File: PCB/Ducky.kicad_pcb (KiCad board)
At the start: 2 copper layers, 34.5 x 94.5 mm, 4 parts, among them J1 Conn_01x22_Socket, J2 Conn_01x22_Socket, U1 ESP32-S3

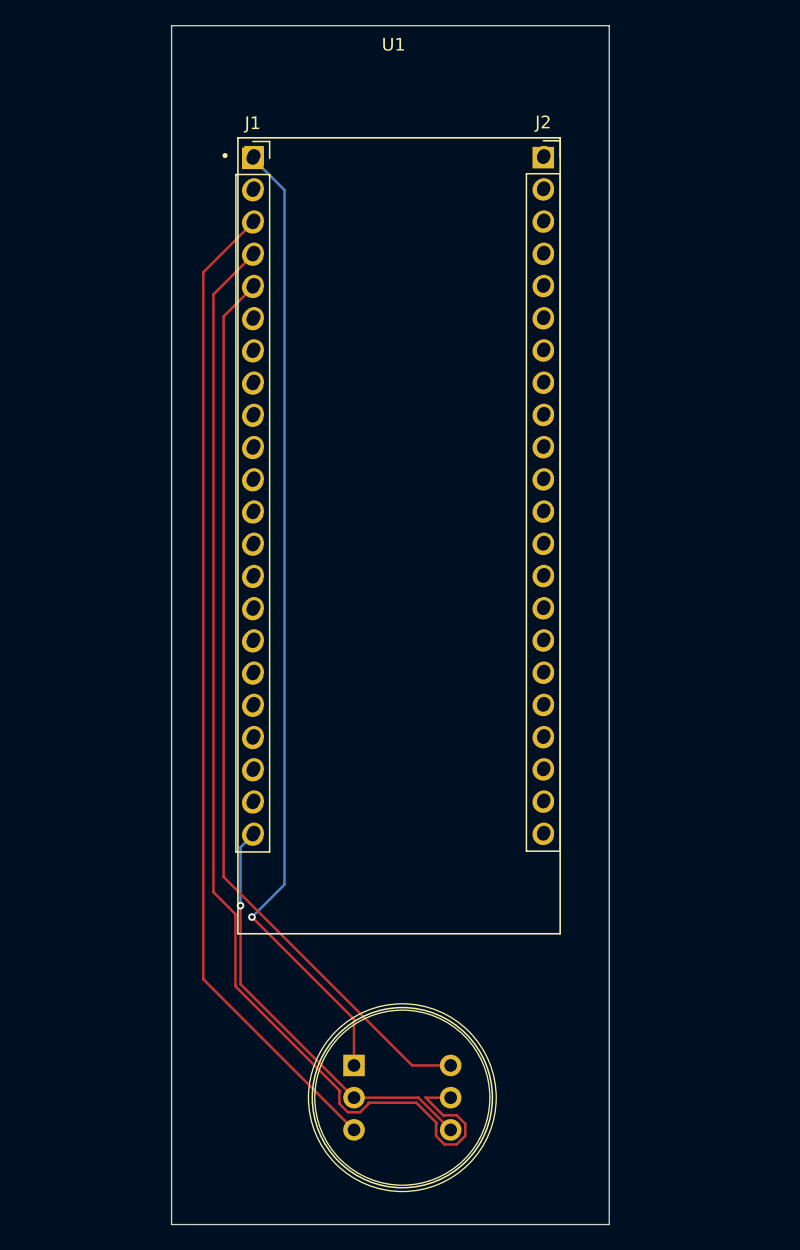
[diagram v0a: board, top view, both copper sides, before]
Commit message: I am organzing my folders and files
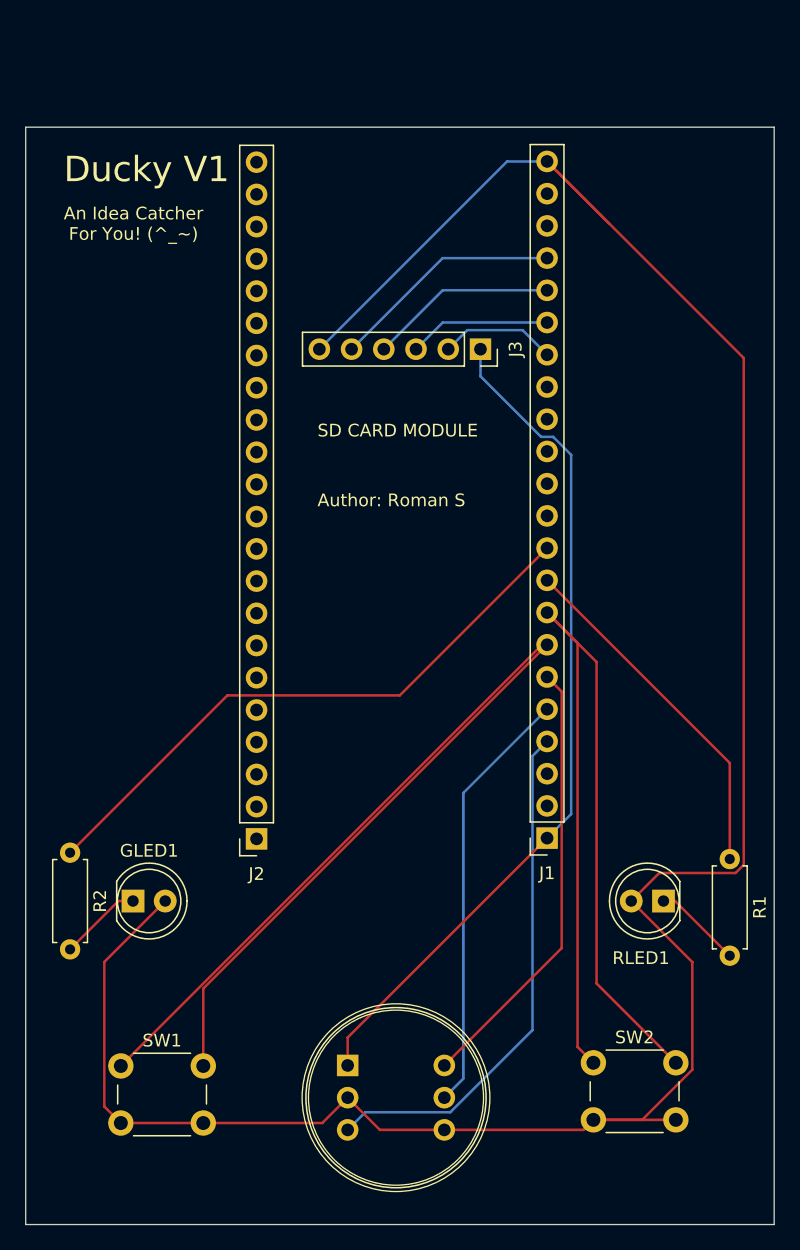
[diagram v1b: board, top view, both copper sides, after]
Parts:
- removed U1: ESP32-S3, ESP32-S3-DEVKITC-1-N8R2:XCVR_ESP32-S3-DEVKITC-1-N8R2
- added GLED1: LED, LED_THT:LED_D5.0mm, F.Cu at (130.5, 97.0)
- added J3: Conn_01x06_Socket, Connector_PinSocket_2.54mm:PinSocket_1x06_P2.54mm_Vertical, F.Cu at (157.8, 53.5)
- added R1: R, Resistor_THT:R_Axial_DIN0207_L6.3mm_D2.5mm_P7.62mm_Horizontal, F.Cu at (177.5, 93.7)
- added R2: R, Resistor_THT:R_Axial_DIN0207_L6.3mm_D2.5mm_P7.62mm_Horizontal, F.Cu at (125.5, 93.2)
- added RLED1: LED, LED_THT:LED_D5.0mm, F.Cu at (172.3, 97.0)
- added SW1: On/Off Button, Button_Switch_THT:SW_PUSH_6mm_H7.3mm, F.Cu at (129.5, 110.0)
- added SW2: Recording/Stop Recording Button, Button_Switch_THT:SW_PUSH_6mm_H7.3mm, F.Cu at (166.8, 109.8)
- moved J1 58.4 mm to (163.1, 92.0), turned to 180 degrees
- moved J2 58.3 mm to (140.2, 92.1), turned to 180 degrees
- moved M1 0.50 mm to (151.2, 112.5)
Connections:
- J1 pad 10: unconnected-(J1-Pin_10-Pad10) -> /GLED
- J1 pad 16: unconnected-(J1-Pin_16-Pad16) -> /CS
- J1 pad 17: unconnected-(J1-Pin_17-Pad17) -> /MOSI
- J1 pad 18: unconnected-(J1-Pin_18-Pad18) -> /CLK
- J1 pad 19: unconnected-(J1-Pin_19-Pad19) -> /MISO
- J1 pad 3: /SD -> unconnected-(J1-Pin_3-Pad3)
- J1 pad 4: /WS -> /SD
- J1 pad 5: /SCK -> /WS
- J1 pad 6: unconnected-(J1-Pin_6-Pad6) -> /SCK
- J1 pad 7: unconnected-(J1-Pin_7-Pad7) -> /On/Off Btn
- J1 pad 8: unconnected-(J1-Pin_8-Pad8) -> /Rec/Stop Btn
- J1 pad 9: unconnected-(J1-Pin_9-Pad9) -> /RLED
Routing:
- net GND: track 33.5 -> 193.6 mm, vias 1 -> 0
- net /On/Off Btn: track 0.00 -> 91.8 mm
- net /Rec/Stop Btn: track 0.00 -> 76.7 mm
- net /WS: track 92.2 -> 34.0 mm
- net /GLED: track 0.00 -> 47.5 mm
- net /SD: track 78.0 -> 41.1 mm
- net /SCK: track 71.5 -> 34.9 mm
- net /RLED: track 0.00 -> 27.9 mm
- net /MISO: track 0.00 -> 18.4 mm
- net /CLK: track 0.00 -> 14.8 mm
- net /MOSI: track 0.00 -> 11.2 mm
- net +3V3: track 76.9 -> 67.3 mm, vias 1 -> 0
- net /CS: track 0.00 -> 9.21 mm
- net Net-(RLED1-K): track 0.00 -> 7.01 mm
- net Net-(GLED1-K): track 0.00 -> 6.54 mm
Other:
- board size 34.5 x 94.5 mm -> 59 x 86.5 mm
- board text added: "An Idea Catcher For You! (^_~)"
- board text added: "M1"
- board text added: "SD CARD MODULE"
- board text removed: "An Idea Catcher For You!"
- board text removed: "INMP441"
